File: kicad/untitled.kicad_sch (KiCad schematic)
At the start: 24 parts, among them J11 Conn_01x02_Socket, J12 Conn_01x02_Socket, J13 AVR-ISP-6, J3 AVR-ISP-6, J4 AVR-ISP-6, J6 Conn_01x01_Pin, J7 Conn_01x01_Pin, J8 Conn_01x01_Pin, J9 Conn_01x01_Pin, M1 Motor_DC, Q1 NMOS, Q2 NMOS, SW4 SW_SPDT, U3 ATmega328P-P, U4 ATmega328P-P, U5 ATmega328P-P

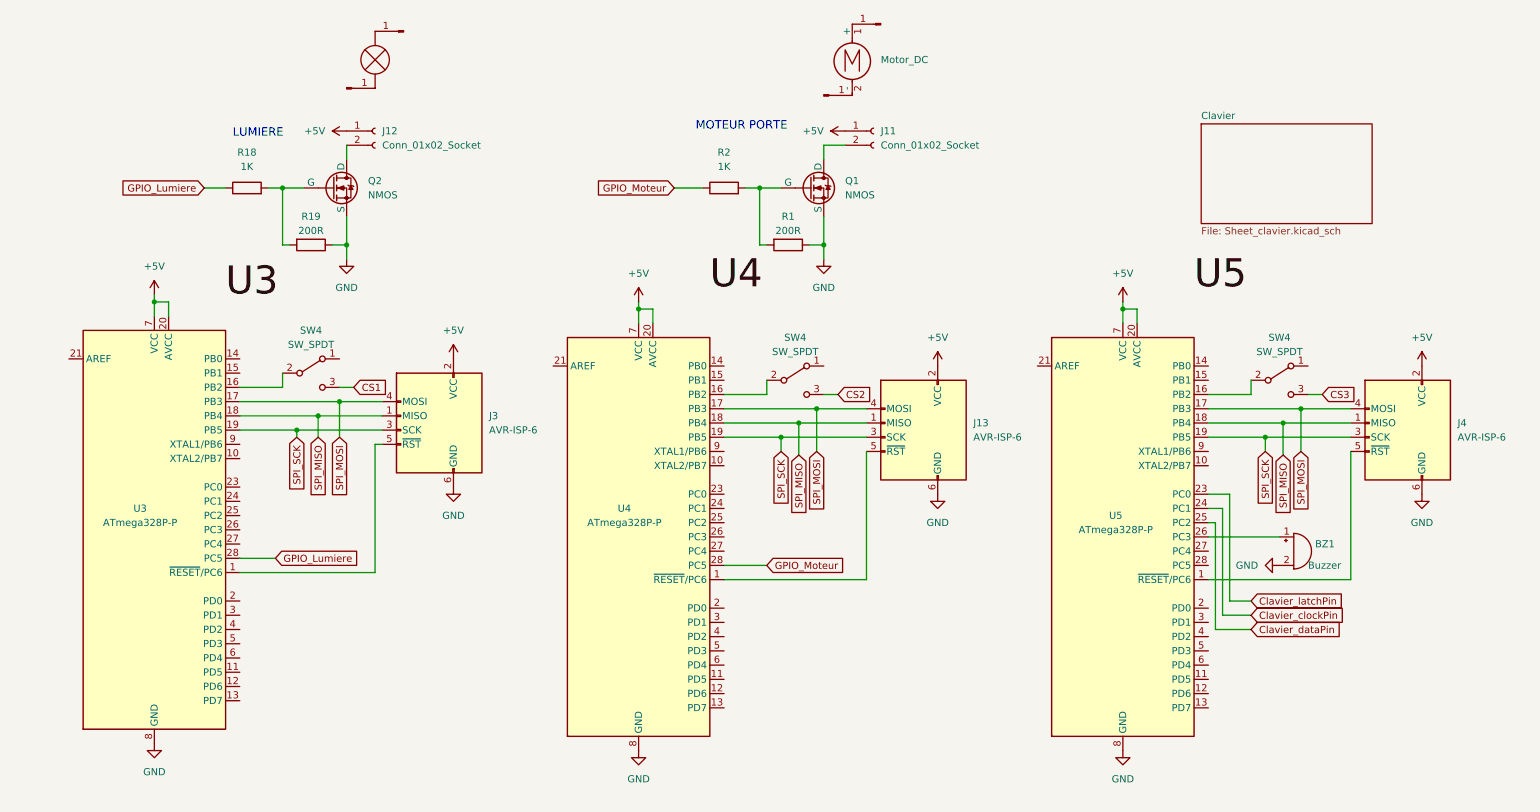
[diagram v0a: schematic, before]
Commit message: 13-10
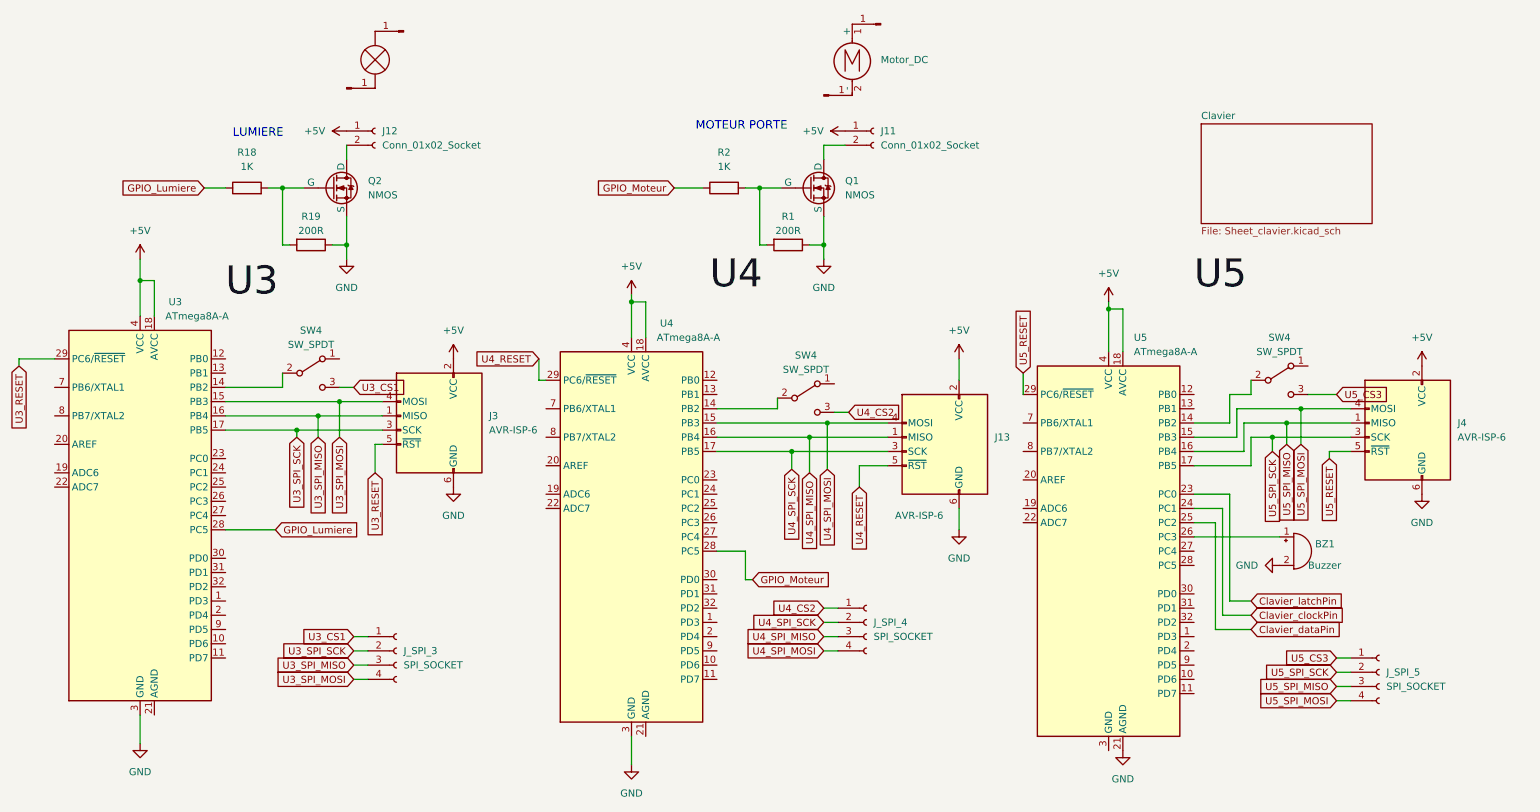
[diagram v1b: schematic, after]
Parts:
- removed U3, U4, U5: ATmega328P-P, Package_DIP:DIP-28_W7.62mm, symbol MCU_Microchip_ATmega:ATmega328P-P
- added J_SPI_3, J_SPI_4, J_SPI_5: SPI_SOCKET, Connector:NS-Tech_Grove_1x04_P2mm_Vertical, symbol Connector:Conn_01x04_Socket
- added U3, U4, U5: ATmega8A-A, Package_QFP:TQFP-32_7x7mm_P0.8mm, symbol MCU_Microchip_ATmega:ATmega8A-A
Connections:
- net +5V: now also U3.18 (AVCC), U3.4 (VCC), U3.6 (VCC), U4.18 (AVCC), U4.4 (VCC), U4.6 (VCC), U5.18 (AVCC), U5.4 (VCC), U5.6 (VCC)
- net Clavier_clockPin: now also U5.24 (PC1)
- net Clavier_dataPin: now also U5.25 (PC2)
- net Clavier_latchPin: now also U5.23 (PC0)
- net GND: now also U3.3 (GND), U3.5 (GND), U4.3 (GND), U4.5 (GND), U5.21 (AGND)
- net GPIO_Lumiere: now also U3.28 (PC5)
- net GPIO_Moteur: now also U4.28 (PC5)
- net at SW4.2 (B): now also U4.14 (PB2)
- net U3_RESET: now reaches J3.5 (~{RST})
- net U3_RESET: now also U3.29 (PC6/~{RESET})
- net at SW4.2 (B): now also U3.14 (PB2)
- net U4_RESET: now reaches J13.5 (~{RST})
- net U4_RESET: now also U4.29 (PC6/~{RESET})
- net U5_RESET: now reaches J4.5 (~{RST})
- net U5_RESET: now also U5.29 (PC6/~{RESET})
- net at BZ1.1 (-): now also U5.26 (PC3)
- net at SW4.2 (B): now also U5.14 (PB2)
- net CS1 renamed U3_CS1
- net U3_CS1: now also J_SPI_3.1 (Pin_1)
- net CS2 renamed U4_CS2
- net U4_CS2: now also J_SPI_4.1 (Pin_1)
- net CS3 renamed U5_CS3
- net U5_CS3: now also J_SPI_5.1 (Pin_1)
- removed net SPI_MISO: J13.1 (MISO), J3.1 (MISO), J4.1 (MISO)
- removed net SPI_MOSI: J13.4 (MOSI), J3.4 (MOSI), J4.4 (MOSI)
- removed net SPI_SCK: J13.3 (SCK), J3.3 (SCK), J4.3 (SCK)
- new net: U5.3 (GND), U5.5 (GND)
- new net U3_SPI_MISO: J3.1 (MISO), J_SPI_3.3 (Pin_3), U3.16 (PB4)
- new net U3_SPI_MOSI: J3.4 (MOSI), J_SPI_3.4 (Pin_4), U3.15 (PB3)
- new net U3_SPI_SCK: J3.3 (SCK), J_SPI_3.2 (Pin_2), U3.17 (PB5)
- new net U4_SPI_MISO: J13.1 (MISO), J_SPI_4.3 (Pin_3), U4.16 (PB4)
- new net U4_SPI_MOSI: J13.4 (MOSI), J_SPI_4.4 (Pin_4), U4.15 (PB3)
- new net U4_SPI_SCK: J13.3 (SCK), J_SPI_4.2 (Pin_2), U4.17 (PB5)
- new net U5_SPI_MISO: J4.1 (MISO), J_SPI_5.3 (Pin_3), U5.16 (PB4)
- new net U5_SPI_MOSI: J4.4 (MOSI), J_SPI_5.4 (Pin_4), U5.15 (PB3)
- new net U5_SPI_SCK: J4.3 (SCK), J_SPI_5.2 (Pin_2), U5.17 (PB5)
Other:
- moved on the sheet: J13, SW4
